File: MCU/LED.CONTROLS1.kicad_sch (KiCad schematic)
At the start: 8 parts, among them U5 HHG1D-1, U7 AMC1301DWVR

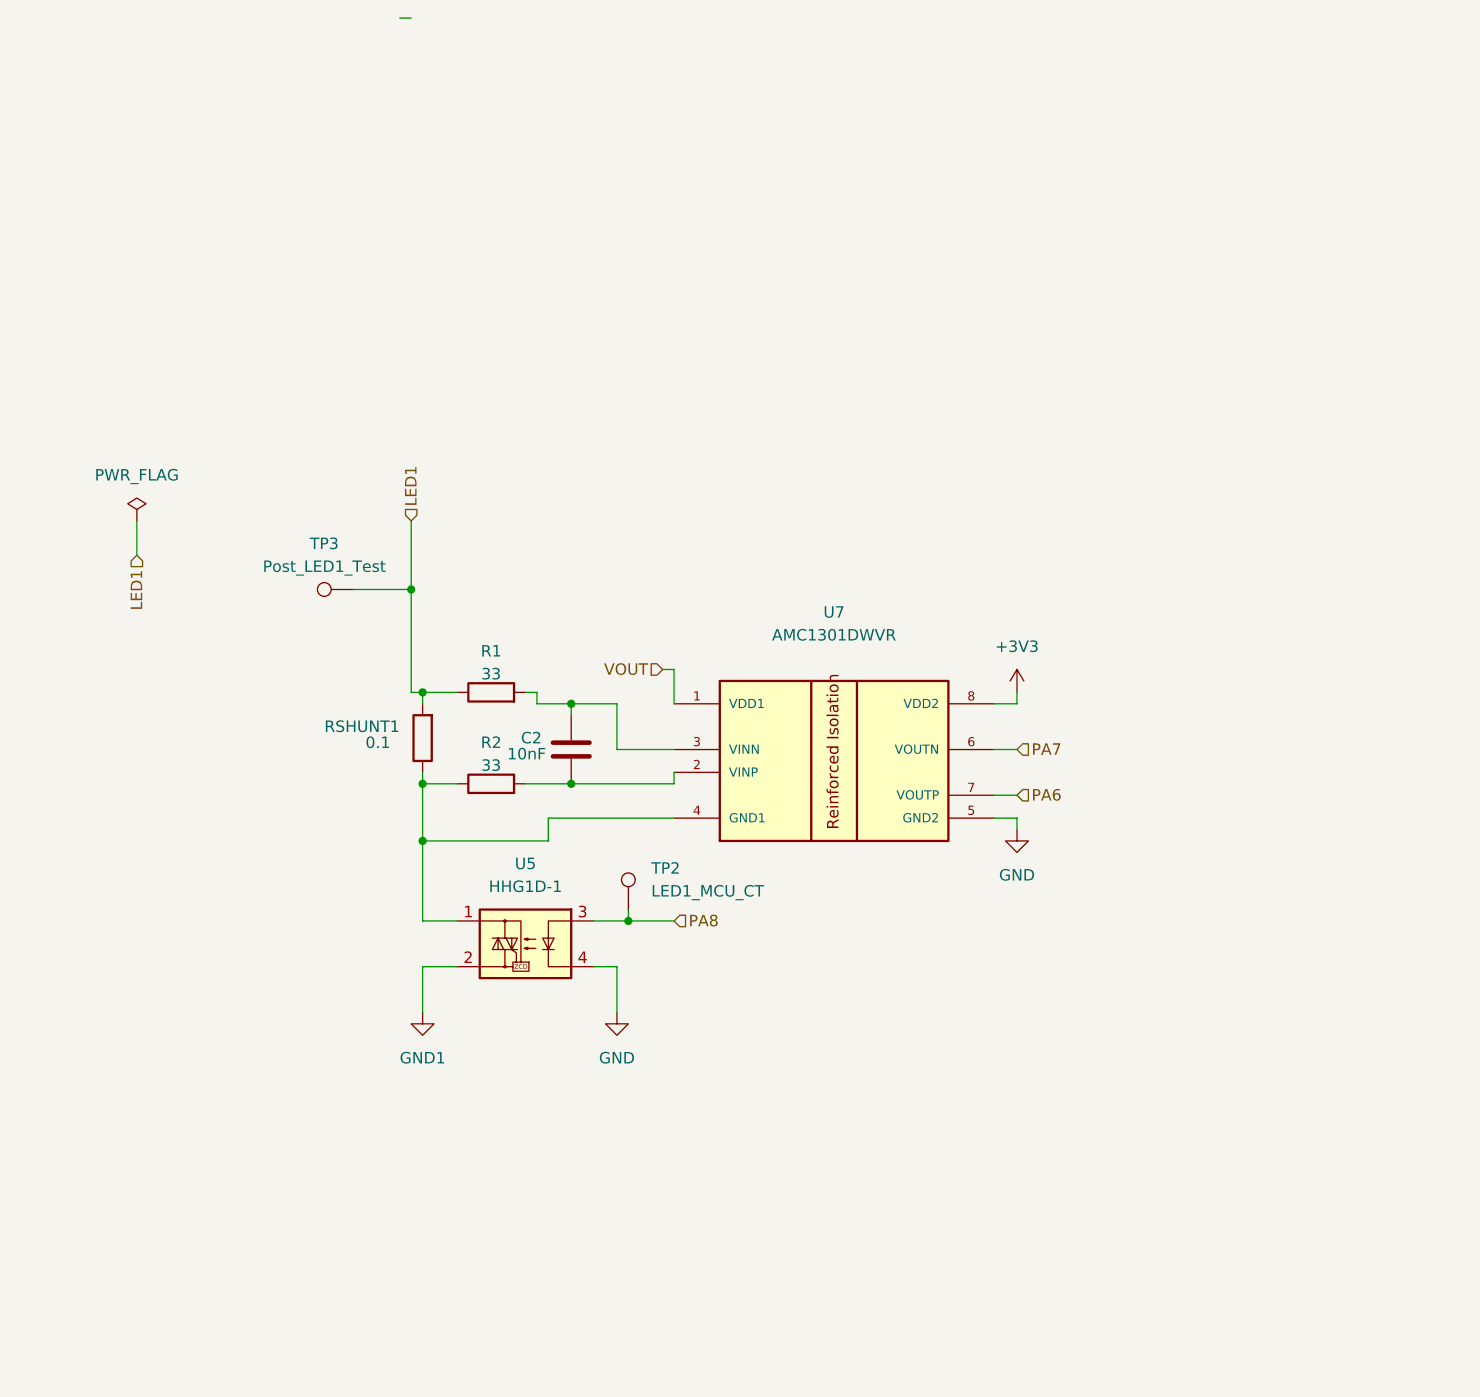
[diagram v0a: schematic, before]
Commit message: Finalized schematic and started layout
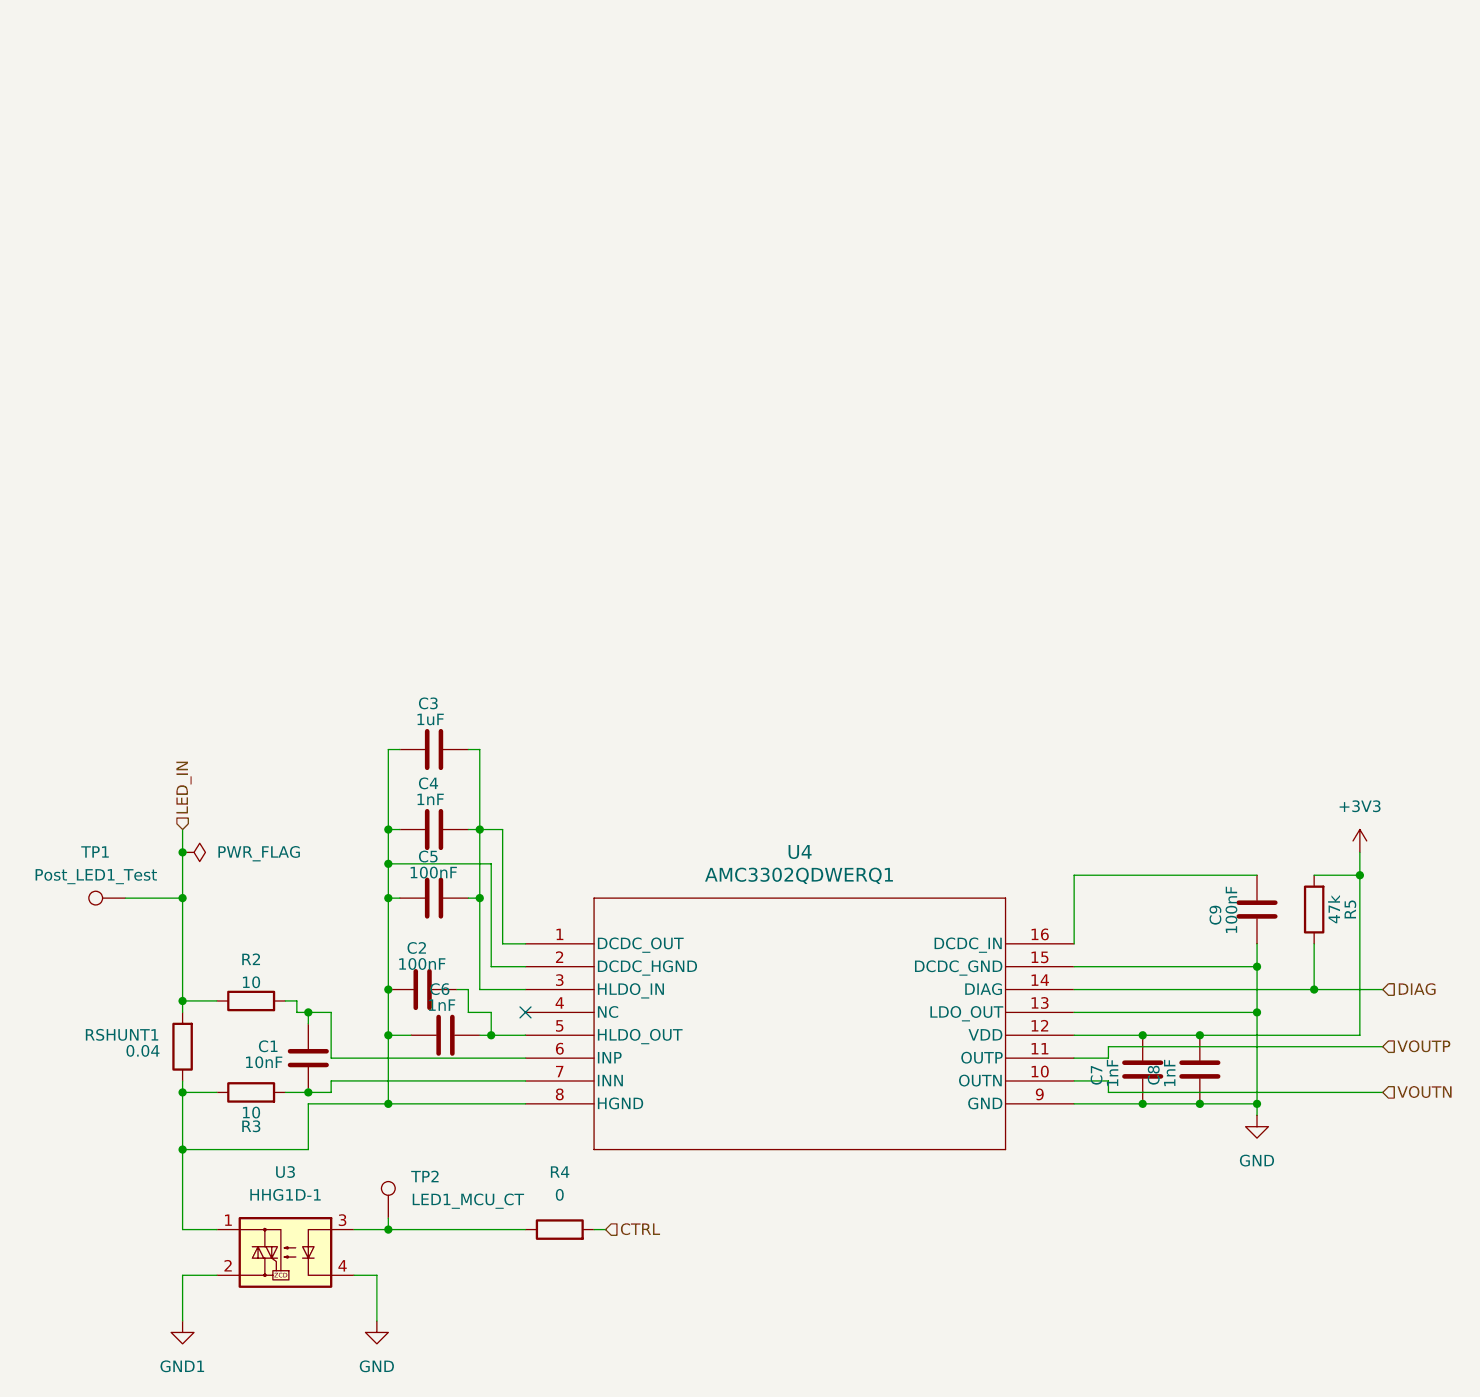
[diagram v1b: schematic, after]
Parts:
- removed R2: 33, Resistor_SMD:R_1812_4532Metric_Pad1.30x3.40mm_HandSolder, symbol Device:R
- removed U7: AMC1301DWVR, AMC1301DWVR:SOIC127P1150X280-8N, symbol AMC1301:AMC1301DWVR
- added C2, C5, C9: 100nF, Capacitor_SMD:C_0201_0603Metric_Pad0.64x0.40mm_HandSolder, symbol Device:C
- added C3: 1uF, Capacitor_SMD:C_0201_0603Metric_Pad0.64x0.40mm_HandSolder, symbol Device:C
- added C4, C6, C7, C8: 1nF, Capacitor_SMD:C_0201_0603Metric_Pad0.64x0.40mm_HandSolder, symbol Device:C
- added R3: 10, Resistor_SMD:R_0603_1608Metric_Pad0.98x0.95mm_HandSolder, symbol Device:R
- added R4: 0, Resistor_SMD:R_0603_1608Metric_Pad0.98x0.95mm_HandSolder, symbol Device:R
- added R5: 47k, Resistor_SMD:R_0603_1608Metric_Pad0.98x0.95mm_HandSolder, symbol Device:R
- added U4: AMC3302QDWERQ1, AMC3302-Q1 Isolated Amplifier:SOIC-3302DWERQ1_TEX, symbol AMC3302-Q1 Isolated Amp:AMC3302QDWERQ1
- R2: renamed from R1; value 33 -> 10; footprint Resistor_SMD:R_1812_4532Metric_Pad1.30x3.40mm_HandSolder -> Resistor_SMD:R_0603_1608Metric_Pad0.98x0.95mm_HandSolder
- RSHUNT1: value 0.1 -> 0.04; footprint Resistor_SMD:R_1812_4532Metric_Pad1.30x3.40mm_HandSolder -> Resistor_SMD:R_2512_6332Metric_Pad1.40x3.35mm_HandSolder
- renumbered C2 to C1, TP3 to TP1, U5 to U3
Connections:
- net +3V3: now also C7.1, C8.1, R5.2, U4.12 (VDD)
- net GND: now also C7.2, C8.2, C9.2, U4.13 (LDO_OUT), U4.15 (DCDC_GND), U4.9 (GND)
- net at C1.1, R2.2: now also U4.6 (INP)
- net at C1.2: now also R3.2, U4.7 (INN)
- net at RSHUNT1.1, U3.1: now also C2.2, C3.2, C4.2, C5.2, C6.2, R3.1, U4.2 (DCDC_HGND), U4.8 (HGND)
- net LED1 renamed LED_IN
- net PA8: no longer names the net of TP2.1, U3.3
- net PA8: now also R4.1
- new net: C3.1, C4.1, C5.1, U4.1 (DCDC_OUT), U4.3 (HLDO_IN)
- new net: C9.1, U4.16 (DCDC_IN)
- new net: C2.1, C6.1, U4.5 (HLDO_OUT)
- new net CTRL: R4.2
- new net DIAG: R5.1, U4.14 (DIAG)
- new net VOUTN: U4.10 (OUTN)
- new net VOUTP: U4.11 (OUTP)
- no-connect marks 0 -> 1
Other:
- moved on the sheet: C1, R2, RSHUNT1, TP1, TP2, U3

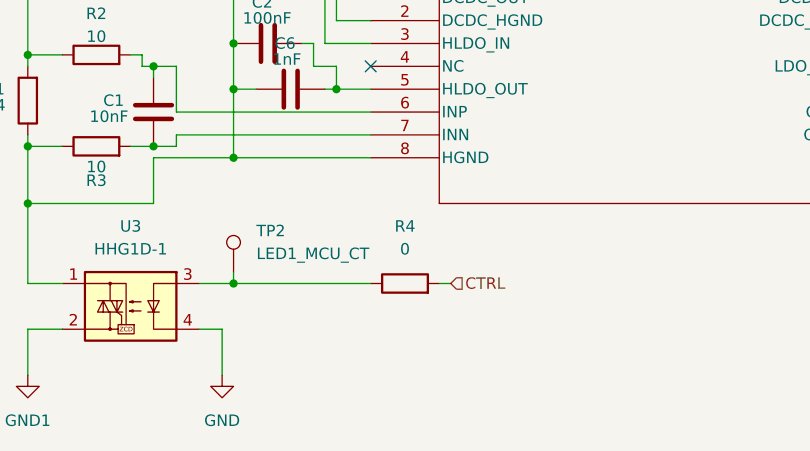
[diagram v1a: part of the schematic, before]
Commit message: MCU Layout V1
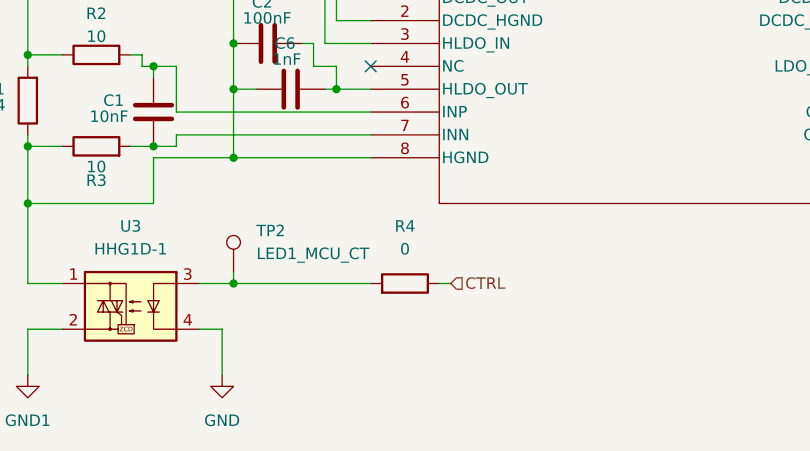
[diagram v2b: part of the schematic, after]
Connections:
- net CTRL: now also R4.1; no longer R4.2
- net at TP2.1, U3.3: now also R4.2; no longer R4.1
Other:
- moved on the sheet: R4
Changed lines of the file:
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@@
 	(symbol
 		(lib_id "Device:R")
-		(at 134.62 118.11 90)
+		(at 134.62 118.11 270)
+		(mirror x)
 		(unit 1)
 		(exclude_from_sim no)
@@
 		(on_board yes)
 		(dnp no)
-		(fields_autoplaced yes)
 		(property "Reference" "R4"
 			(at 134.62 111.76 90)
